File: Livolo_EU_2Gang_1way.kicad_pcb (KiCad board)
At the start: 2 copper layers, 43 x 43 mm, 39 parts, among them IC1 ATMEGA328P, U1 ATSHA204A, U2 RFM69_MINIMAL

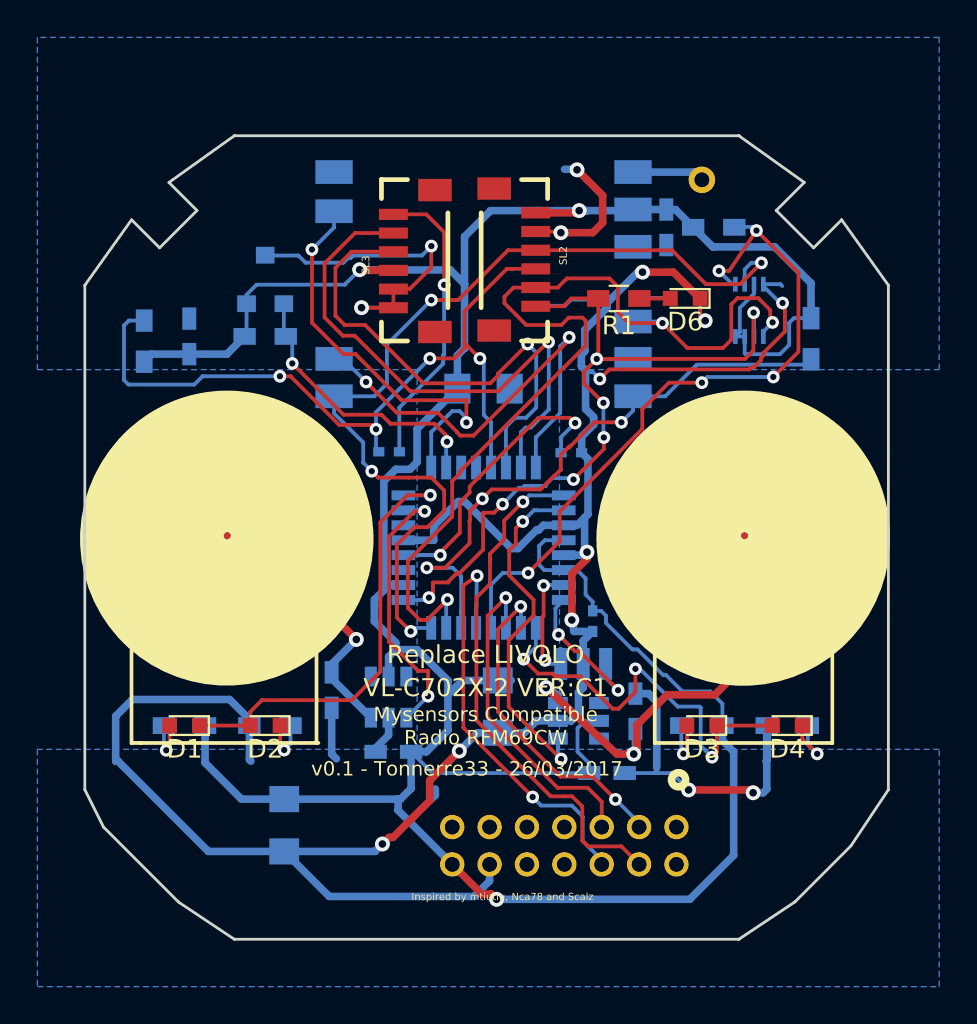
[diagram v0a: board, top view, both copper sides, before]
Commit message: update gerber
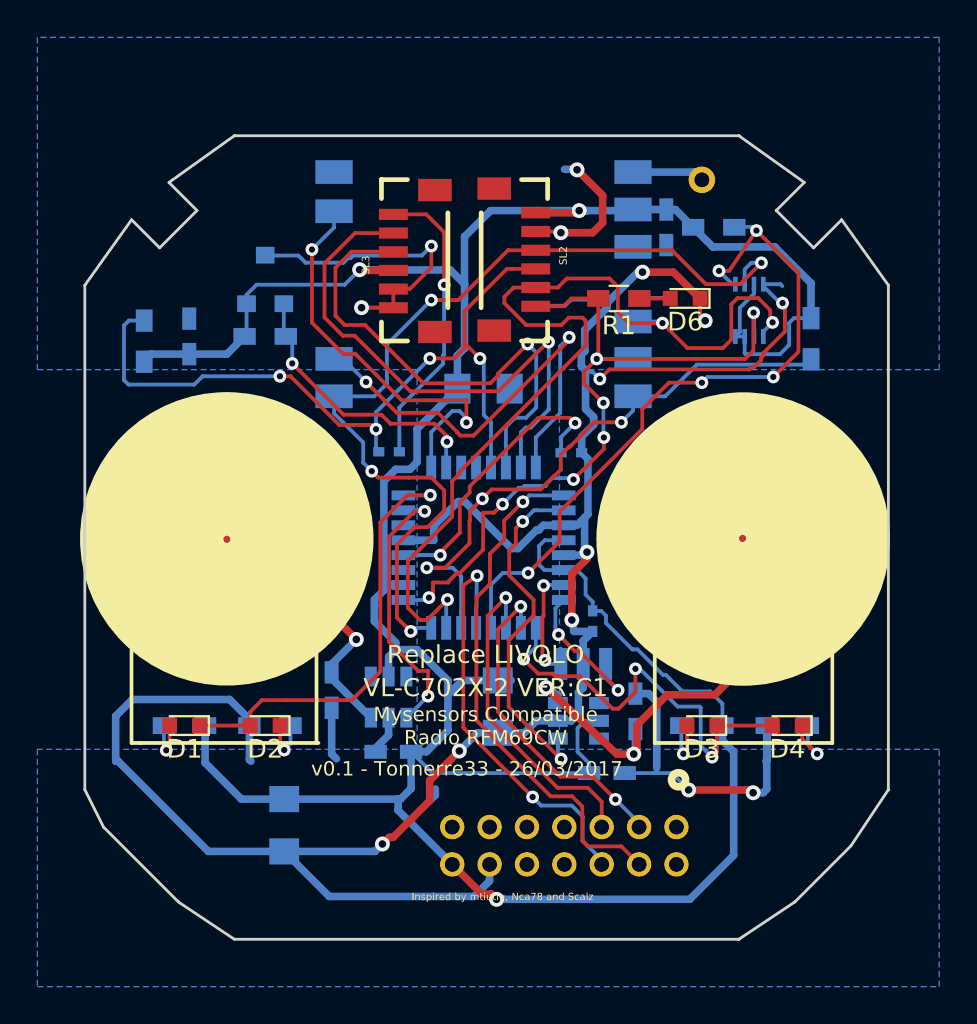
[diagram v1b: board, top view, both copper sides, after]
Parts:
- moved U$5 0.19 mm to (134.6, 105.1)
- moved U$1 0.18 mm to (162.2, 105.0)
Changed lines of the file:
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@@
     (links 100)
     (no_connects 0)
-    (area 126.926099 83.428599 170.076101 126.578601)
+    (area 124.46 78.24 172.720001 139.426629)
     (thickness 1.6)
     (drawings 35)
@@
   )
   (module Livolo:touch_pad_16mm (layer Bottom)
-    (at 134.62 104.91)
+    (at 134.6 105.1)
     (fp_text reference U$5 (at -0.075 -0.85) (layer B.SilkS) hide
       (effects (font (size 0.4 0.4) (thickness 0.1)) (justify mirror))
@@
   )
   (module Livolo:touch_pad_16mm (layer Bottom)
-    (at 162.306 104.91)
+    (at 162.2 105.05)
     (fp_text reference U$1 (at -0.075 -0.85) (layer B.SilkS) hide
       (effects (font (size 0.4 0.4) (thickness 0.1)) (justify mirror))
